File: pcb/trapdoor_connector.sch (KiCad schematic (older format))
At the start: 1 part, among them X1 A1200_trapdoor_connector

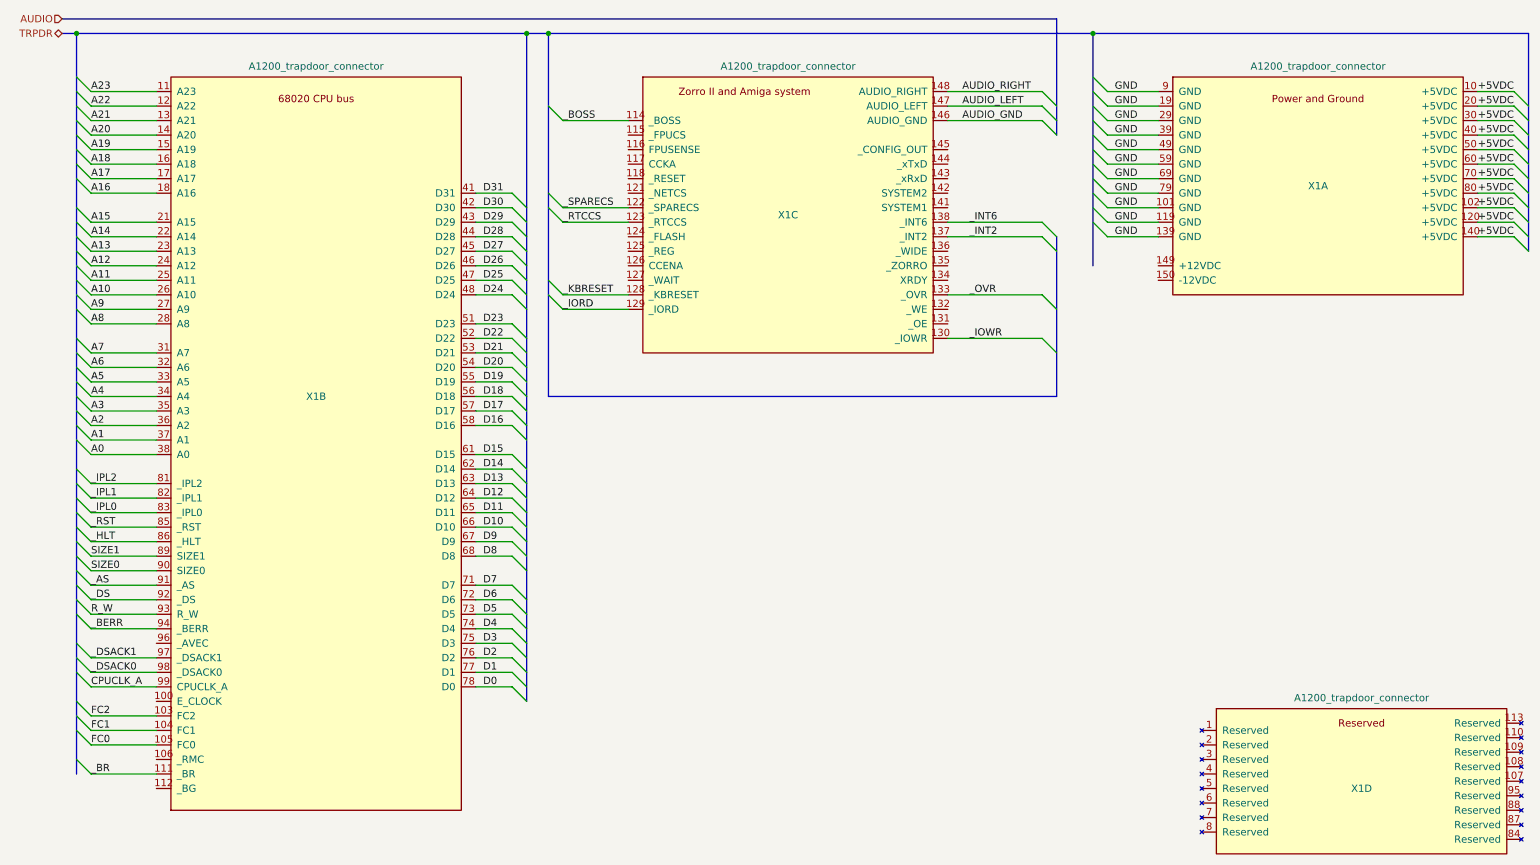
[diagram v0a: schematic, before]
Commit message: some work on sheets
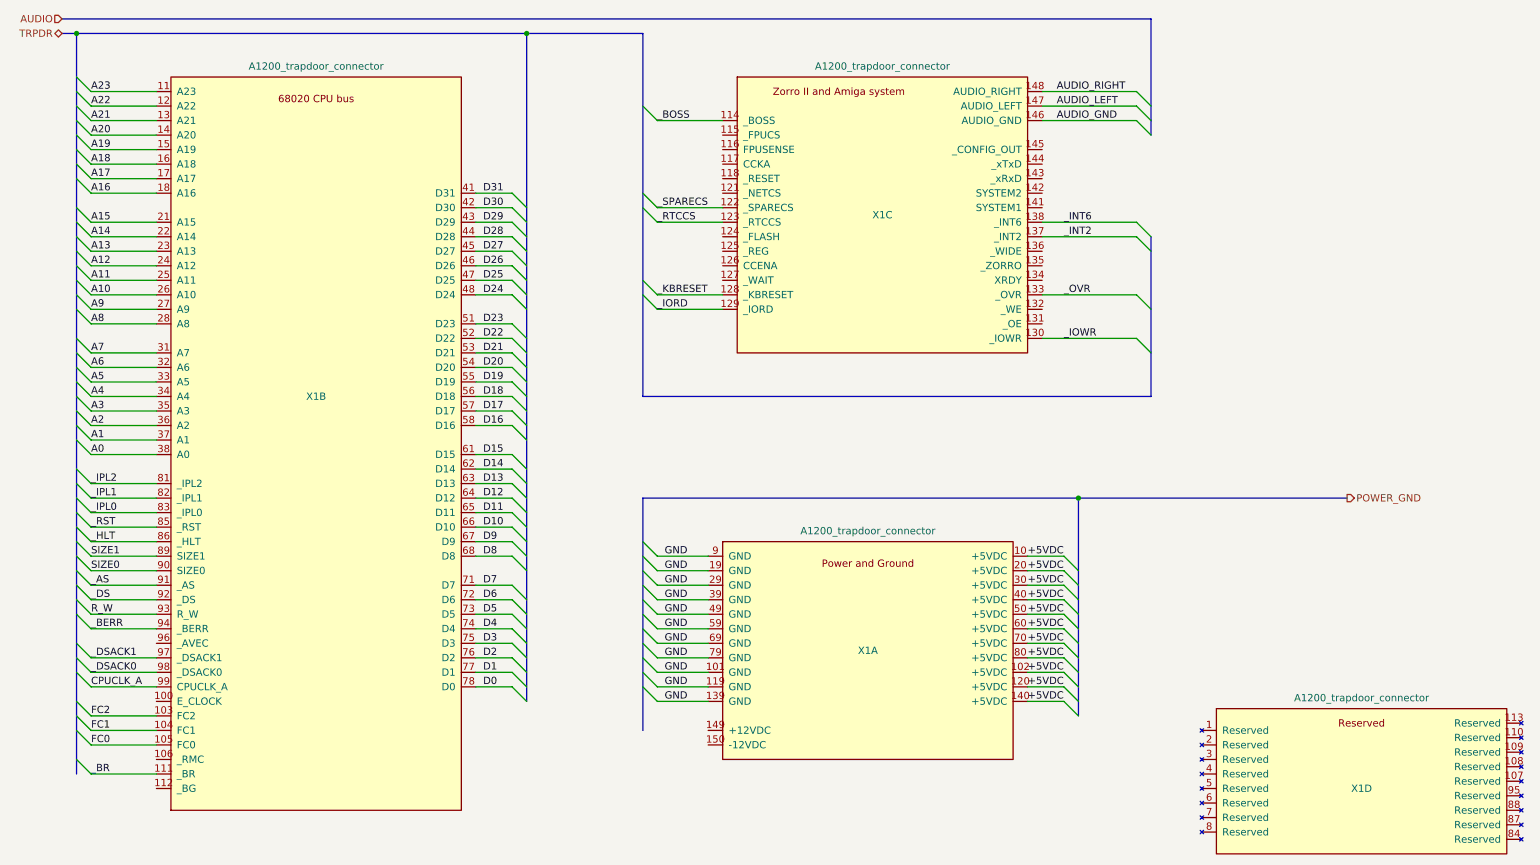
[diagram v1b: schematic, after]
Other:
- moved on the sheet: X1A, X1C
